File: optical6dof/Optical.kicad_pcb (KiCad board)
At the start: 4 copper layers, 7.3 x 7.3 mm, 16 parts, among them U1 MAX11617EWE+T

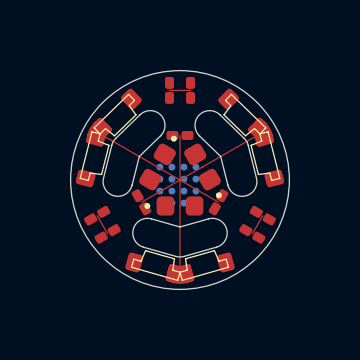
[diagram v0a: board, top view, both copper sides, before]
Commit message: routed the pcb
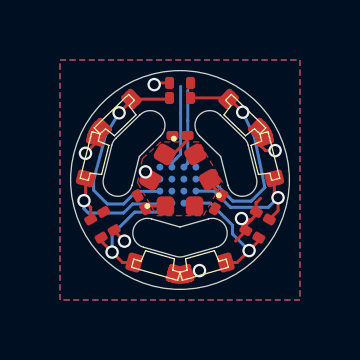
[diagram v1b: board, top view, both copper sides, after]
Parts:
- turned R2 to 90 degrees
- turned R5 to 90 degrees
- turned R7 to 180 degrees
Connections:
- U1 pad A1: unconnected-(U1-AIN0-PadA1) -> /A1
- U1 pad A2: unconnected-(U1-AIN1-PadA2) -> /B2
- U1 pad A4: unconnected-(U1-AIN3-PadA4) -> /B1
- U1 pad B1: unconnected-(U1-AIN9-PadB1) -> /A2
- U1 pad B4: unconnected-(U1-AIN4-PadB4) -> /C2
- U1 pad C4: unconnected-(U1-AIN5-PadC4) -> /C1
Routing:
- net /C1: track 0.00 -> 7.36 mm, vias 0 -> 1
- net /A2: track 0.00 -> 7.25 mm, vias 0 -> 1
- net /C2: track 0.00 -> 4.64 mm, vias 0 -> 1
- net /B2: track 0.00 -> 4.58 mm, vias 0 -> 1
- net /A1: track 0.00 -> 4.48 mm, vias 0 -> 1
- net /B1: track 0.00 -> 4.11 mm, vias 0 -> 1
- net VDD: track 0.00 -> 3.42 mm, vias 0 -> 4
- net GND: track 0.00 -> 3.16 mm, vias 0 -> 3
- net /SCL: track 0.00 -> 2.81 mm
- net /SDA: track 0.00 -> 2.62 mm
- net Net-(D1-K): track 0.00 -> 1.11 mm
- net Net-(D2-K): track 0.00 -> 0.71 mm
- net Net-(D3-K): track 0.00 -> 0.71 mm
- added copper zone on B.Cu, net GND
- added copper zone on F.Cu, net GND
- added copper zone on In1.Cu, net GND
- added copper zone on F.Cu, net VDD
- added copper zone on In2.Cu, net VDD
